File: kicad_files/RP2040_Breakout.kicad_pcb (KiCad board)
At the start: 2 copper layers, 21 x 51 mm, 56 parts, among them IC1 RPI_Chip_RP2040-10-10, IC2 RT6150B-33GQW, IC3 W25Q16JVUXIQ_TR, J1 690-005-298-486, J2 Conn_02x20_Counter_Clockwise, J3 Conn_01x03_Pin, Q1 DMG1012T-7, Y1 Crystal_GND23

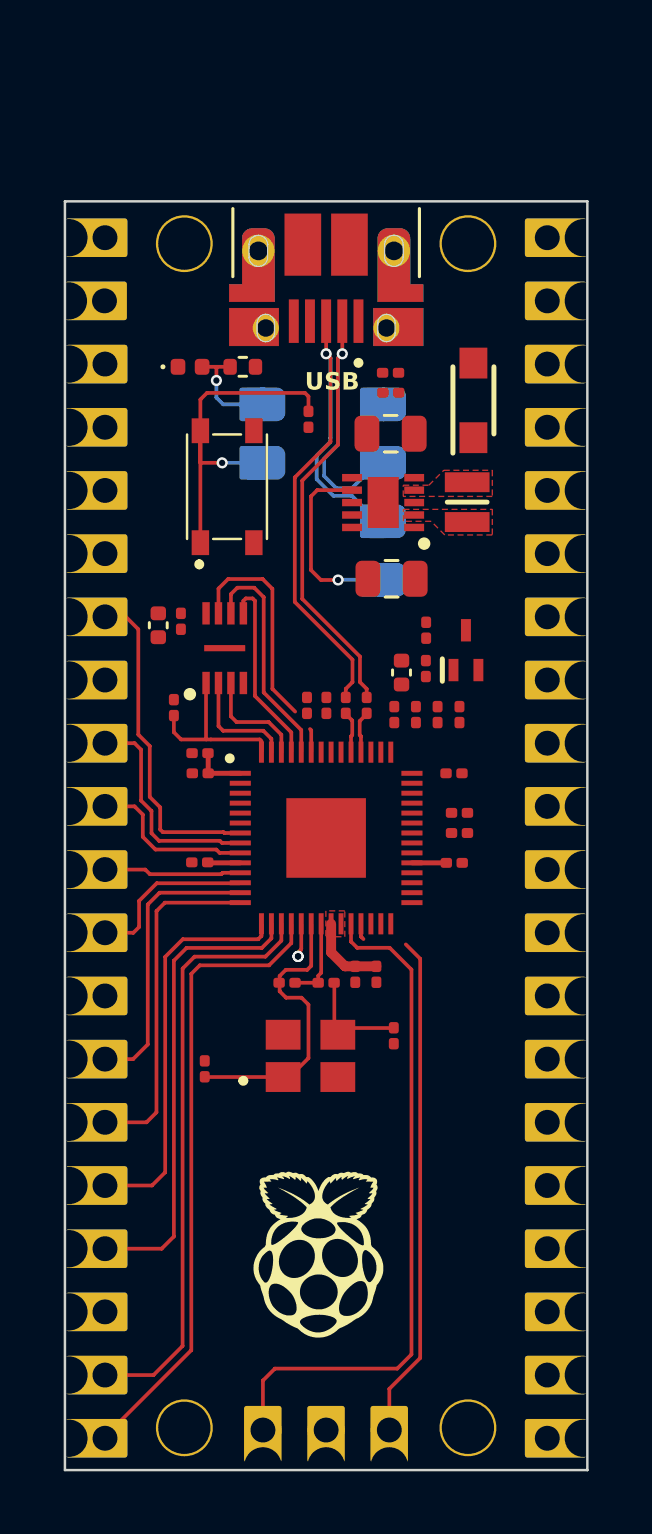
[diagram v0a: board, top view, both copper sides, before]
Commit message: routing progess
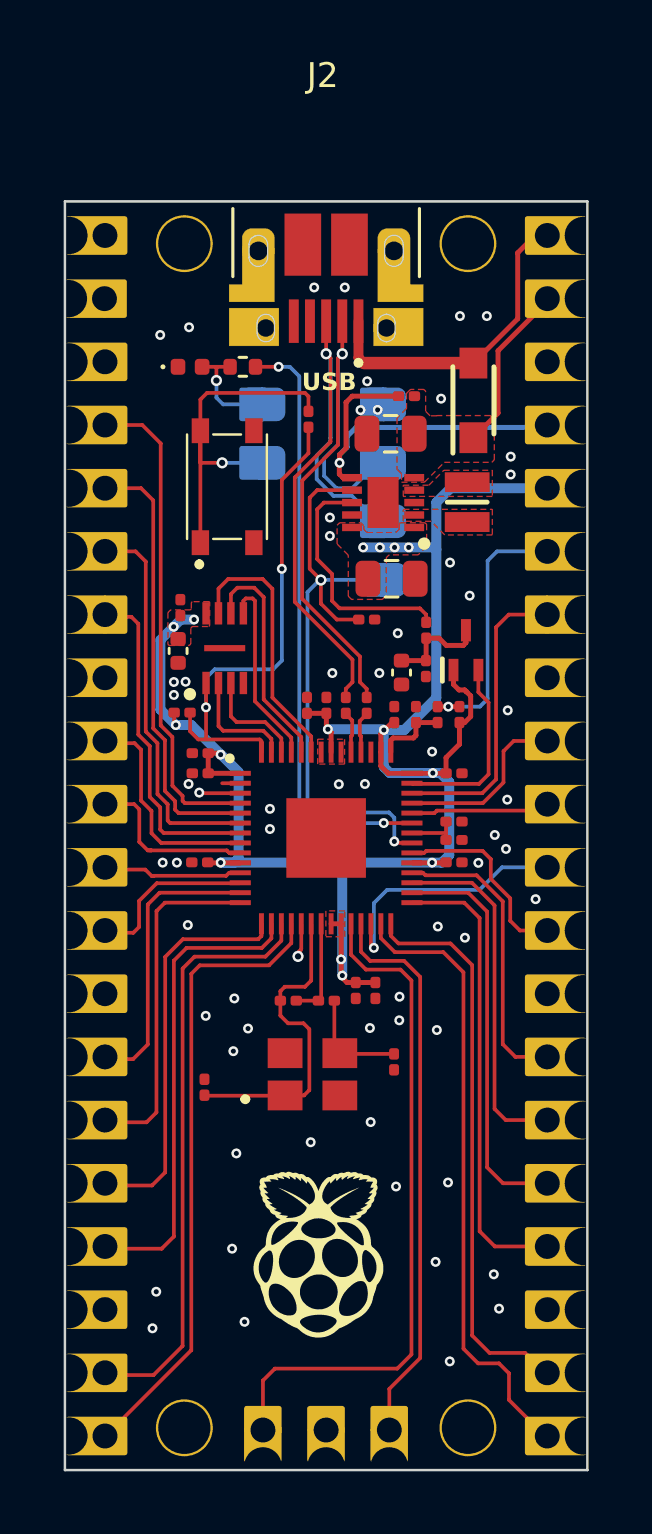
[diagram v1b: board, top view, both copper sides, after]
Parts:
- moved R4 9.17 mm to (138.8, 91.8)
- moved C17 1.30 mm to (131.2, 93.1)
- moved R3 1.14 mm to (140.4, 82.8)
- moved C14 1.05 mm to (139.9, 109.6)
- moved Y1 0.74 mm to (136.6, 110.1)
- moved C13 0.74 mm to (132.2, 110.6)
- moved R7 0.72 mm to (135.6, 107.2)
- moved R8 0.72 mm to (137.1, 107.2)
- moved C6 0.65 mm to (139.1, 106.7)
- moved C2 0.65 mm to (138.3, 106.7)
- moved C16 0.55 mm to (131.3, 91.3), turned to 90 degrees
- moved R1 0.41 mm to (142.3, 100.0)
- moved R13 0.39 mm to (131.3, 95.6), turned to 180 degrees
- moved R2 0.36 mm to (142.3, 100.7)
- moved J2 0.09 mm to (137.1, 100.5)
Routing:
- net /rp2040/DVDD_1: track 8.01 -> 77.8 mm, vias 0 -> 15
- net /rp2040/GPIO16: track 0.00 -> 25.1 mm
- net /rp2040/GPIO25: track 0.00 -> 24.0 mm, vias 0 -> 2
- net /rp2040/GPIO17: track 0.00 -> 22.8 mm
- net /rp2040/GPIO2: track 0.00 -> 19.6 mm
- net /rp2040/GPIO18: track 0.00 -> 18.5 mm
- net /rp2040/GPIO3: track 0.00 -> 17.6 mm
- net /rp2040/GPIO23: track 7.80 -> 25.2 mm, vias 1 -> 2
- net /power_chain/VSYS: track 0.00 -> 16.6 mm
- net /rp2040/GPIO19: track 0.00 -> 16.3 mm
- net /rp2040/GPIO4: track 0.00 -> 15.5 mm
- net /power_chain/3V3_EN: track 0.00 -> 15.2 mm, vias 0 -> 1
- net /rp2040/GPIO20: track 0.00 -> 14.2 mm
- net /rp2040/QSPI_SS_N: track 7.05 -> 20.8 mm, vias 0 -> 2
- net /power_chain/VBUS: track 0.00 -> 12.8 mm
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- added copper zone on F.Cu, net /power_chain/VSYS
